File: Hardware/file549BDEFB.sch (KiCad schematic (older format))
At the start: 46 parts, among them IC1 L293D, K3 I2C, SW10 5, SW11 6, SW12 7, SW13 8, SW14 1, SW15 2, SW16 3, SW17 4, SW2 C, SW3 D, SW4 E, SW5 F, SW6 9, SW7 0, SW8 A, SW9 B, U2 24C16, U3 DS1307, U4 BATTERY, X1 CRYSTAL

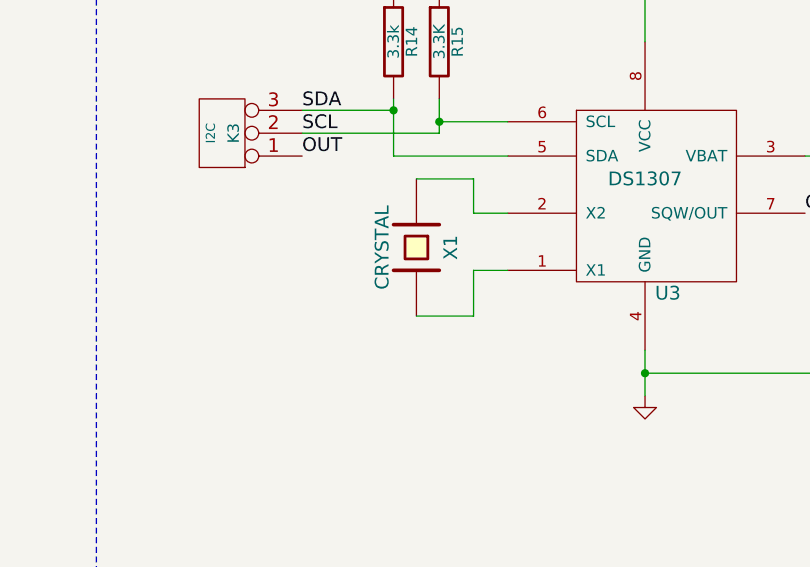
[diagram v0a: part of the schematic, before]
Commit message: added new files
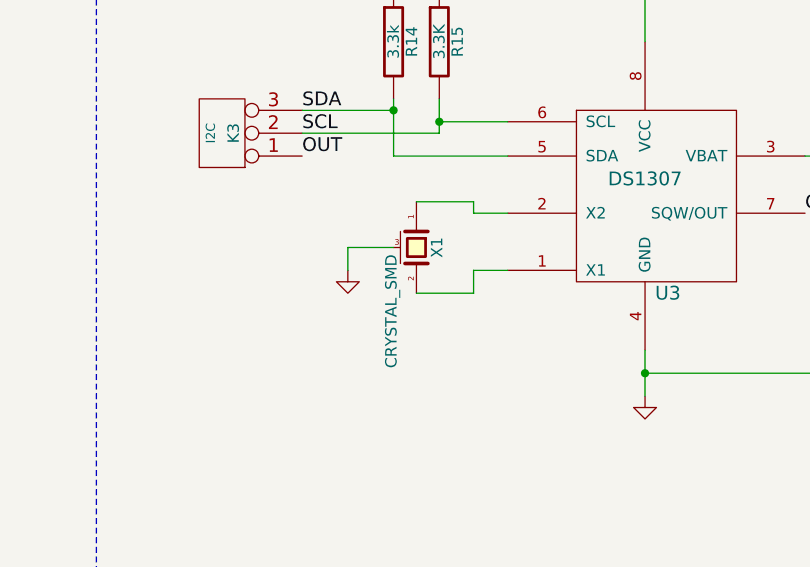
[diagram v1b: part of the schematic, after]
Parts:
- removed X1: CRYSTAL, symbol CRYSTAL
- added X1: CRYSTAL_SMD, symbol CRYSTAL_SMD
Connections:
- net GND: now also X1.3 (case)
- net at U3.2 (X2): now also X1.1
- net at U3.1 (X1): now also X1.2
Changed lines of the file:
@@
 LIBS:contrib
 LIBS:valves
+LIBS:Ultra_DB_X51_v1-cache
+LIBS:16X2-cache
+LIBS:blutooth-cache
 LIBS:MCU_BaseBoard-cache
 EELAYER 25 0
@@
 $EndComp
 $Comp
-L GND #PWR013
+L GND #PWR012
 U 1 1 549BE143
 P 3050 2200
-F 0 "#PWR013" H 3050 2200 30  0001 C CNN
+F 0 "#PWR012" H 3050 2200 30  0001 C CNN
 F 1 "GND" H 3050 2130 30  0001 C CNN
 F 2 "" H 3050 2200 60  0001 C CNN
@@
 M1c
 $Comp
-L GND #PWR014
+L GND #PWR013
 U 1 1 549BE1B9
 P 8400 5500
-F 0 "#PWR014" H 8400 5500 30  0001 C CNN
+F 0 "#PWR013" H 8400 5500 30  0001 C CNN
 F 1 "GND" H 8400 5430 30  0001 C CNN
 F 2 "" H 8400 5500 60  0001 C CNN
@@
 $EndComp
 $Comp
-L GND #PWR015
+L GND #PWR014
 U 1 1 549BE1BF
 P 9600 5500
-F 0 "#PWR015" H 9600 5500 30  0001 C CNN
+F 0 "#PWR014" H 9600 5500 30  0001 C CNN
 F 1 "GND" H 9600 5430 30  0001 C CNN
 F 2 "" H 9600 5500 60  0001 C CNN
@@
 $EndComp
 $Comp
-L CRYSTAL X1
-U 1 1 549BE1D9
-P 5150 2550
-F 0 "X1" H 5150 2700 60  0000 C CNN
-F 1 "CRYSTAL" H 5150 2400 60  0000 C CNN
-F 2 "" H 5150 2550 60  0001 C CNN
-F 3 "" H 5150 2550 60  0001 C CNN
-	1    5150 2550
-	0    1    1    0
-$EndComp
-$Comp
 L BATTERY U4
 U 1 1 549BE1DF
@@
 $EndComp
 $Comp
-L GND #PWR016
+L GND #PWR015
 U 1 1 549BE209
 P 10400 3500
-F 0 "#PWR016" H 10400 3500 30  0001 C CNN
+F 0 "#PWR015" H 10400 3500 30  0001 C CNN
 F 1 "GND" H 10400 3430 30  0001 C CNN
 F 2 "" H 10400 3500 60  0001 C CNN
@@
 $EndComp
 $Comp
-L GND #PWR017
+L GND #PWR016
 U 1 1 549BE245
 P 2350 2900
-F 0 "#PWR017" H 2350 2900 30  0001 C CNN
+F 0 "#PWR016" H 2350 2900 30  0001 C CNN
 F 1 "GND" H 2350 2830 30  0001 C CNN
 F 2 "" H 2350 2900 60  0001 C CNN
@@
 $EndComp
 $Comp
-L GND #PWR018
+L GND #PWR017
 U 1 1 549BE24B
 P 6150 3200
-F 0 "#PWR018" H 6150 3200 30  0001 C CNN
+F 0 "#PWR017" H 6150 3200 30  0001 C CNN
 F 1 "GND" H 6150 3130 30  0001 C CNN
 F 2 "" H 6150 3200 60  0001 C CNN
@@
 	5400 2650 5550 2650
 Wire Wire Line
-	5400 2850 5400 2650
-Wire Wire Line
-	5150 2850 5400 2850
-Wire Wire Line
 	5400 2400 5550 2400
-Wire Wire Line
-	5400 2250 5400 2400
-Wire Wire Line
-	5150 2250 5400 2250
 Connection ~ 6150 3100
 Wire Wire Line
@@
 Wire Bus Line
 	7400 4000 7400 6550
+$Comp
+L CRYSTAL_SMD X1
+U 1 1 55655673
+P 5150 2550
+F 0 "X1" H 5150 2640 50  0000 C CNN
+F 1 "CRYSTAL_SMD" H 5180 2440 50  0000 L CNN
+F 2 "" H 5150 2550 60  0000 C CNN
+F 3 "" H 5150 2550 60  0000 C CNN
+	1    5150 2550
+	0    1    1    0
+$EndComp
+Wire Wire Line
+	5400 2400 5400 2350
+Wire Wire Line
+	5400 2350 5150 2350
+Wire Wire Line
+	5400 2650 5400 2750
+Wire Wire Line
+	5400 2750 5150 2750
+$Comp
+L GND #PWR018
+U 1 1 556562A6
+P 4850 2650
+F 0 "#PWR018" H 4850 2650 30  0001 C CNN
+F 1 "GND" H 4850 2580 30  0001 C CNN
+F 2 "" H 4850 2650 60  0001 C CNN
+F 3 "" H 4850 2650 60  0001 C CNN
+	1    4850 2650
+	1    0    0    -1
+$EndComp
+Wire Wire Line
+	5050 2550 4850 2550
+Wire Wire Line
+	4850 2550 4850 2650
 $EndSCHEMATC
